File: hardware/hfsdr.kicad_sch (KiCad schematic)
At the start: 24 parts, among them J1 USB_C_Receptacle_USB2.0_16P, SW1 RST, SW2 BOOT0, U3 CH32V30xRxTx

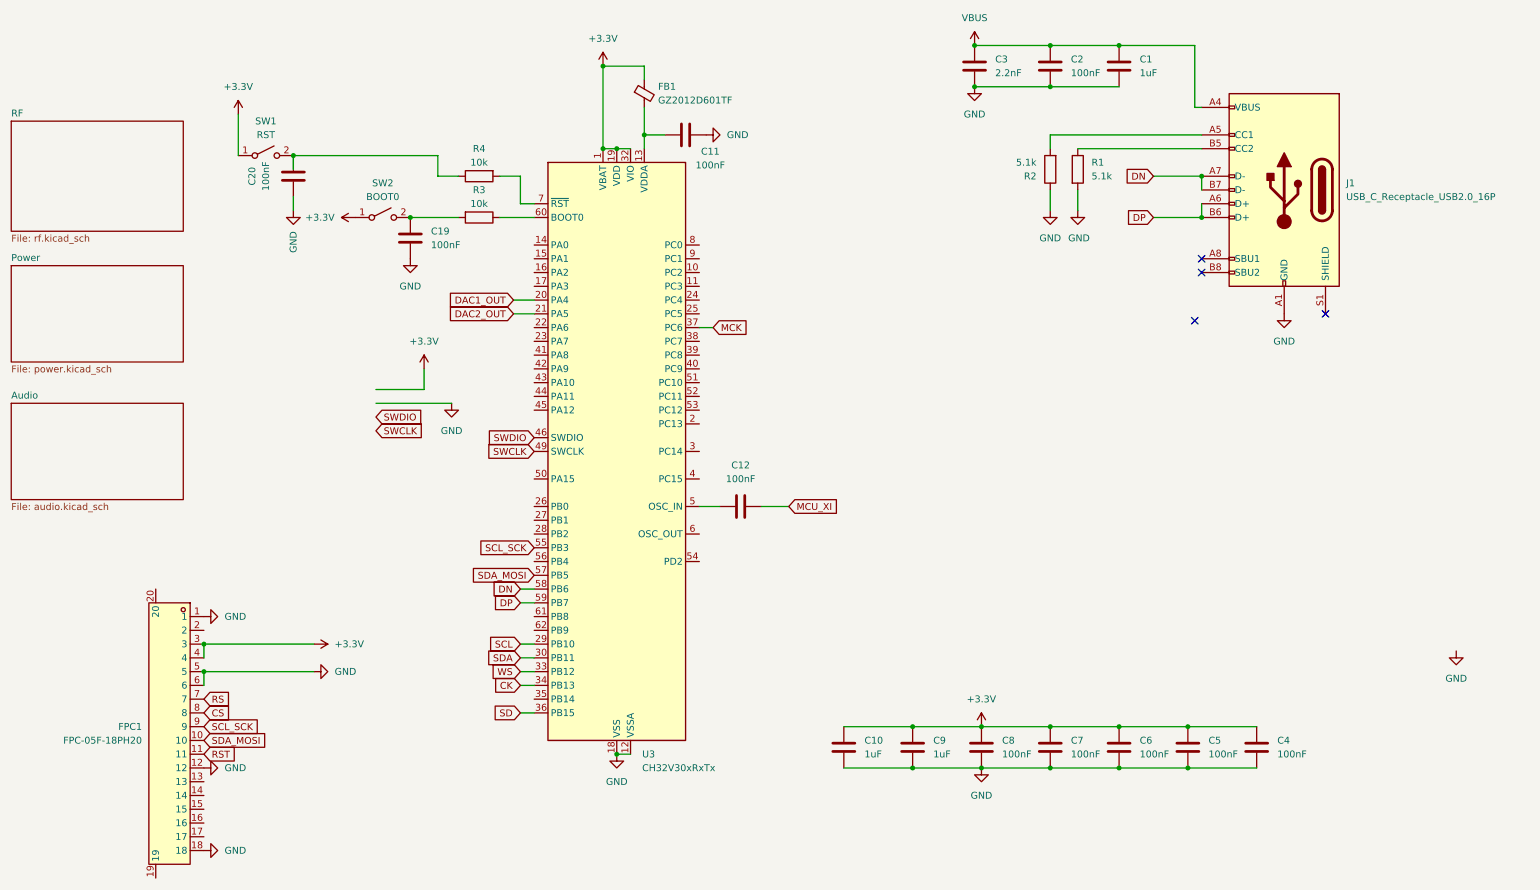
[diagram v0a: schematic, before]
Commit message: feat: hfsdr rough
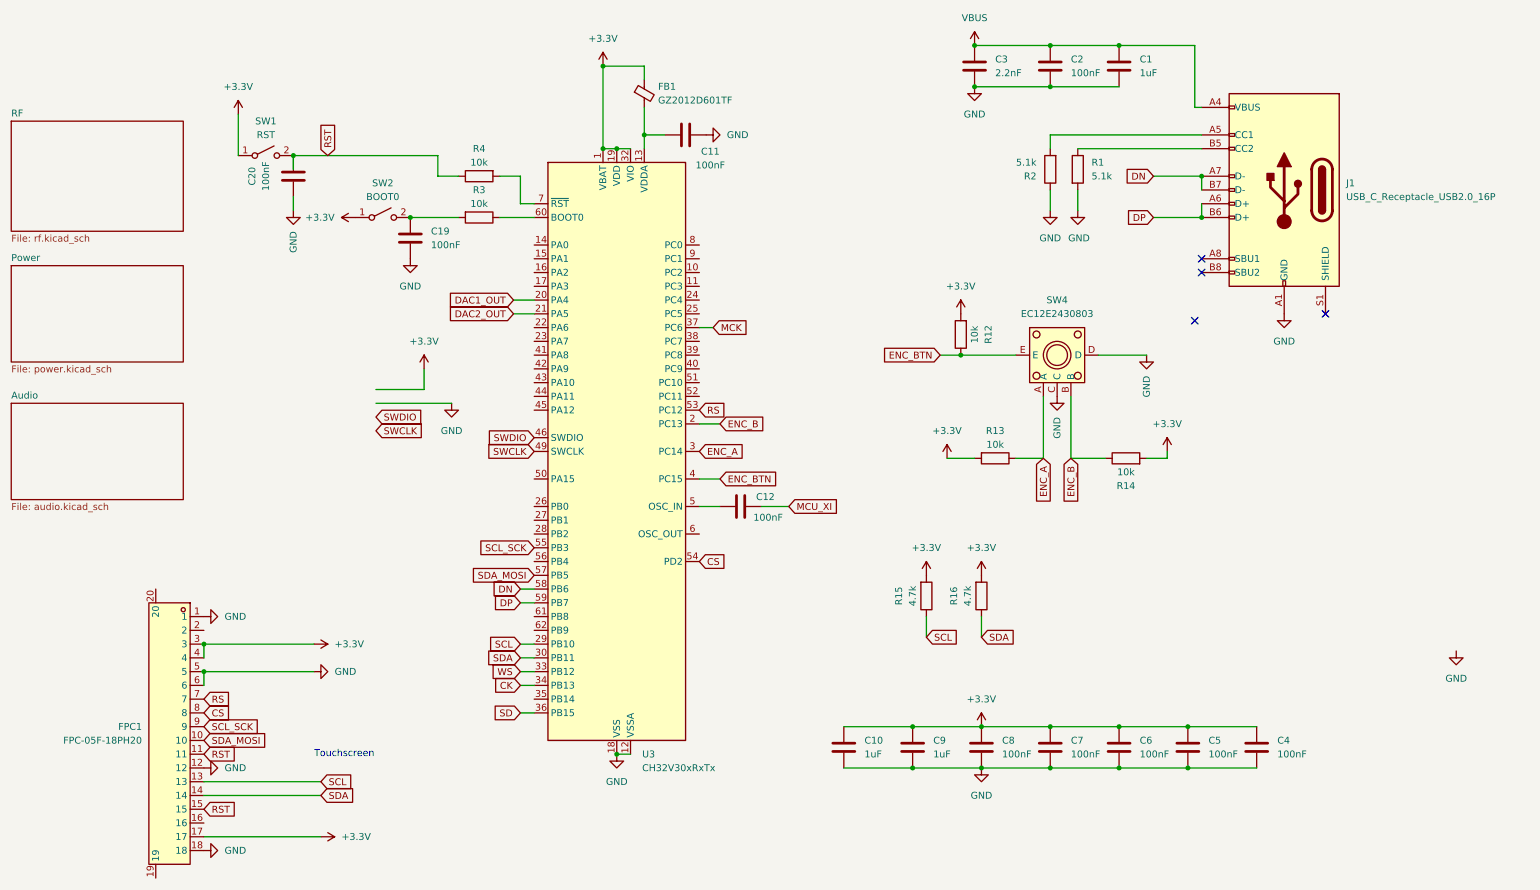
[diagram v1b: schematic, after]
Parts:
- added R12, R13, R14: 10k, Resistor_SMD:R_0805_2012Metric_Pad1.20x1.40mm_HandSolder, symbol Device:R
- added R15, R16: 4.7k, Resistor_SMD:R_0805_2012Metric_Pad1.20x1.40mm_HandSolder, symbol Device:R
- added SW4: EC12E2430803, easyeda2kicad:SW-TH_EC12EXXXX, symbol easyeda2kicad:EC12E2430803
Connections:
- net +3.3V: now also FPC1.17, R12.2, R13.2, R14.2, R15.2, R16.2
- net CS: now also U3.54 (PD2)
- net GND: now also SW4.C, SW4.D
- net RS: now also U3.53 (PC12)
- net RST: now also C20.2, FPC1.15, R4.1, SW1.2 (B)
- net SCL: now also FPC1.13, R15.1
- net SDA: now also FPC1.14, R16.1
- net ENC_B: now reaches U3.2 (PC13)
- net ENC_B: now also R14.1, SW4.B
- net ENC_A: now reaches U3.3 (PC14)
- net ENC_A: now also R13.1, SW4.A
- net ENC_BTN: now reaches U3.4 (PC15)
- net ENC_BTN: now also R12.1, SW4.E
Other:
- note added: "Touchscreen"
